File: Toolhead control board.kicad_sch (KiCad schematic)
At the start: 28 parts, among them J1 Conn_01x02_Pin, J2 Conn_01x02_Pin, J3 Conn_01x06_Pin, J4 Conn_01x02_Pin, J5 Conn_01x02_Pin, J6 Conn_01x02_Pin, Q1 AS3400, Q2 AS3400, Q3 AS3400, U1 ADXL345, U2 STM32F042G6Ux, Y1 8MHz

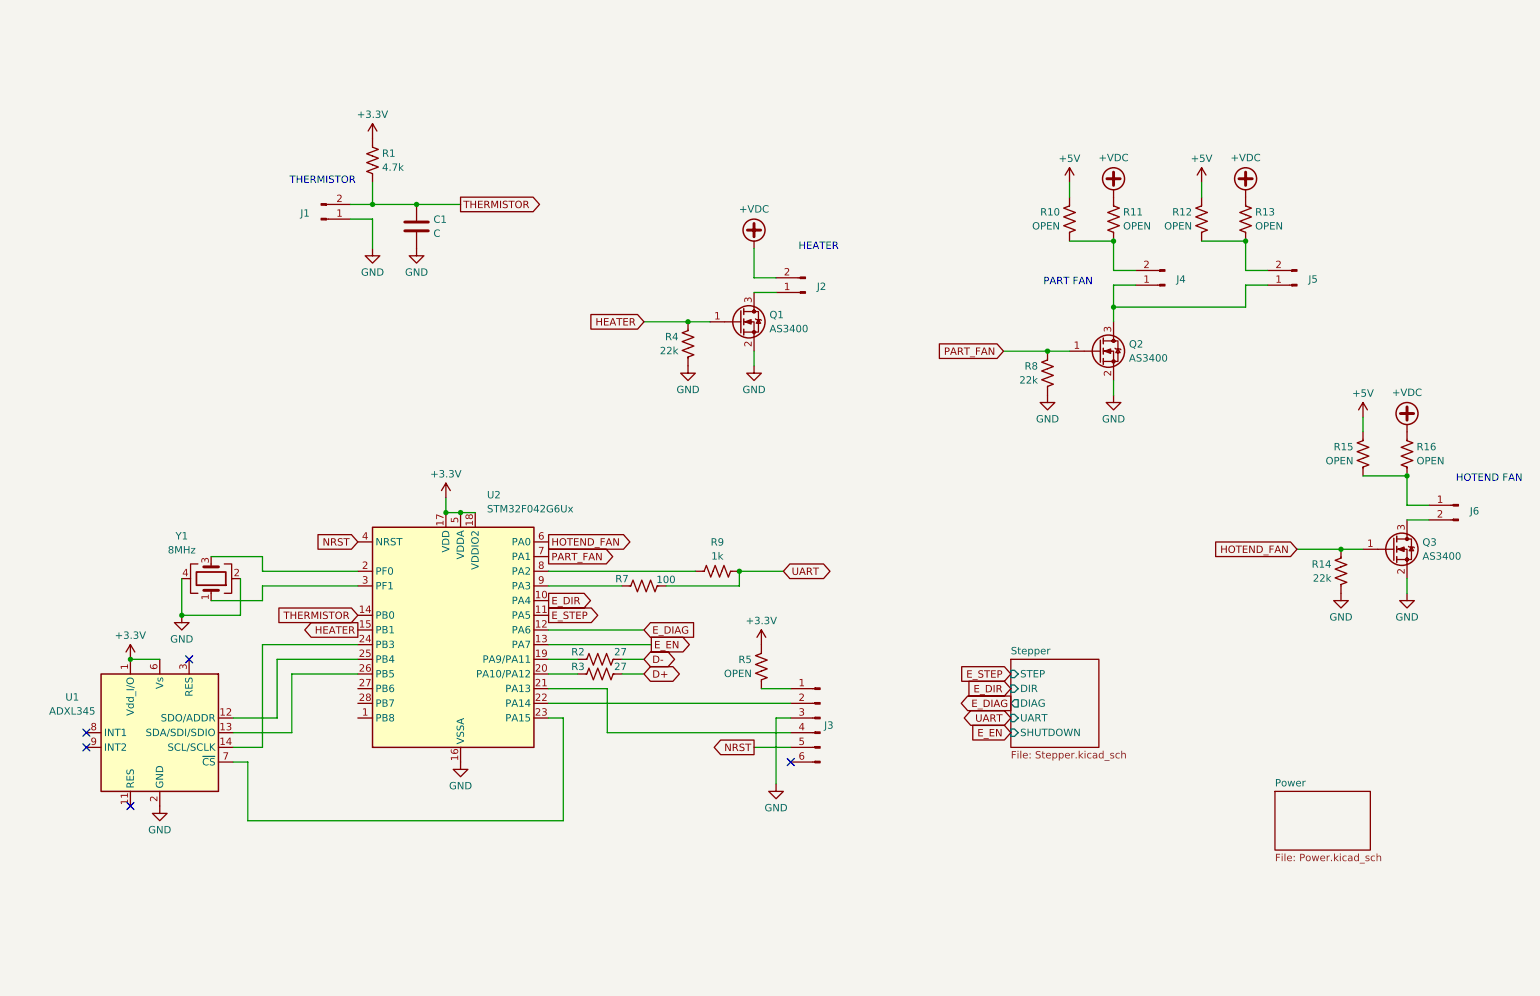
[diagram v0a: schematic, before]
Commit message: Rev1. Uart interface
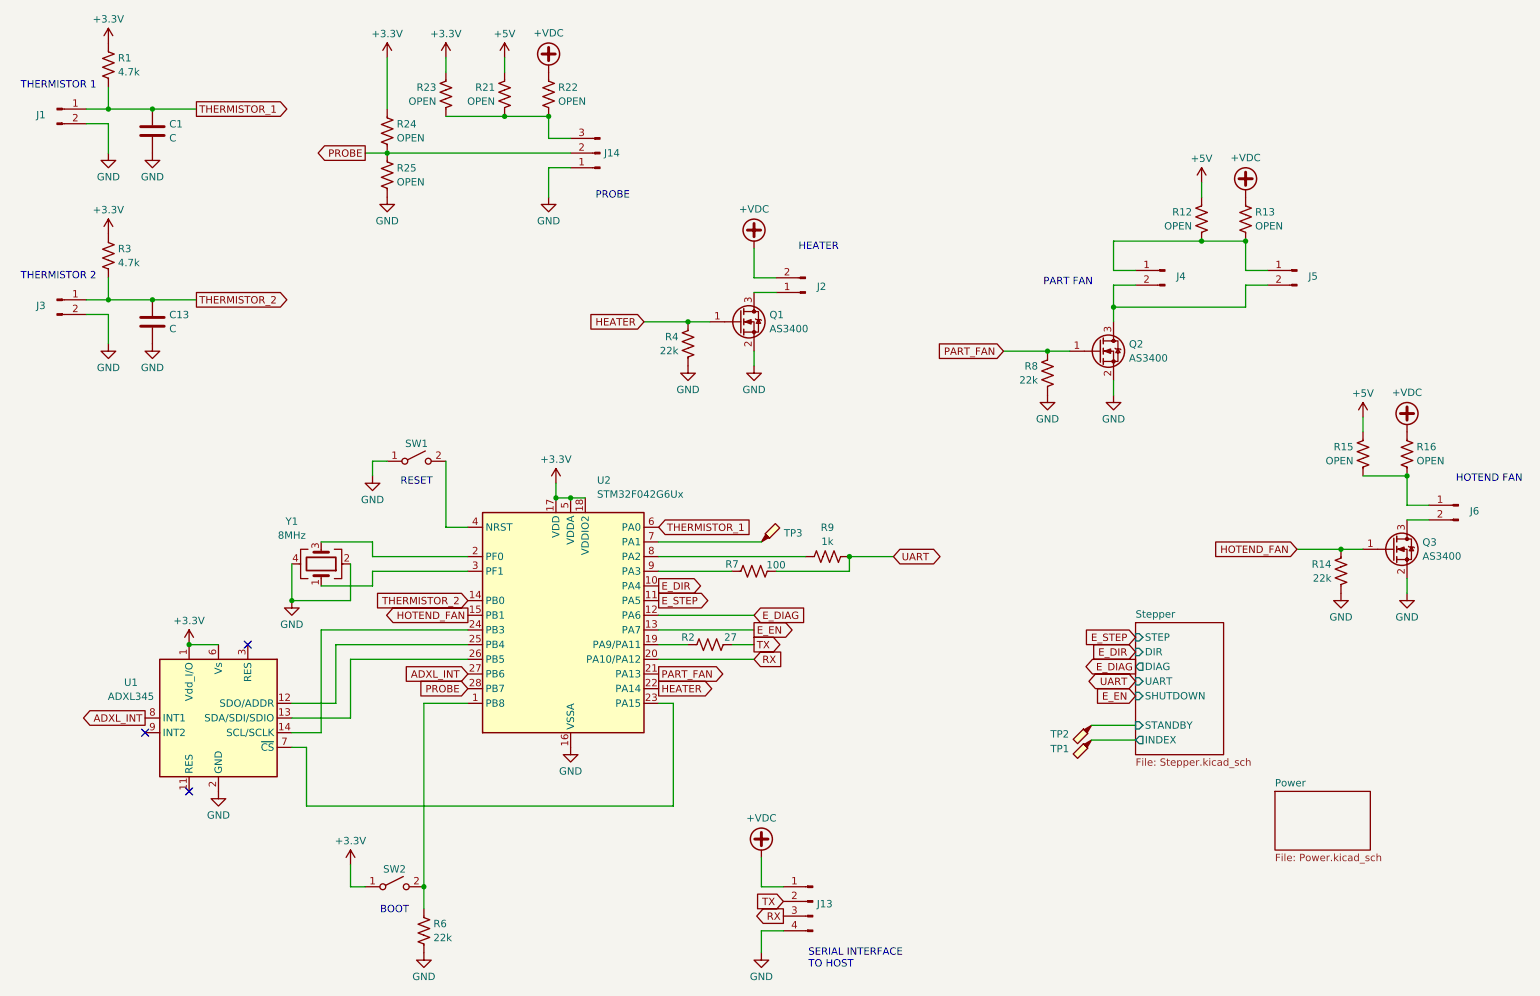
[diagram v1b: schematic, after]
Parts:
- removed J3: Conn_01x06_Pin, Connector_PinHeader_2.54mm:PinHeader_1x06_P2.54mm_Vertical, symbol Connector:Conn_01x06_Pin
- removed R10, R11, R5: OPEN, Resistor_SMD:R_0805_2012Metric, symbol Device:R_US
- added C13: C, Capacitor_SMD:C_0805_2012Metric, symbol Device:C
- added J13: Conn_01x04_Male, Connector_JST:JST_XH_B4B-XH-A_1x04_P2.50mm_Vertical, symbol Connector:Conn_01x04_Male
- added J14: Conn_01x04_Male, Connector_JST:JST_XH_B4B-XH-A_1x04_P2.50mm_Vertical, symbol Connector:Conn_01x03_Pin
- added J3: Conn_01x02_Pin, Connector_JST:JST_XH_S2B-XH-A-1_1x02_P2.50mm_Horizontal, symbol Connector:Conn_01x02_Pin
- added R21, R22, R23, R24, R25: OPEN, Resistor_SMD:R_0805_2012Metric, symbol Device:R_US
- added R6: 22k, Resistor_SMD:R_0805_2012Metric, symbol Device:R_US
- added SW1, SW2: SW_SPST, Button_Switch_SMD:SW_SPST_B3U-1000P, symbol Switch:SW_SPST
- added TP1, TP2, TP3: TestPoint_Probe, TestPoint:TestPoint_Pad_D1.0mm, symbol Connector:TestPoint_Probe
- R3: value 27 -> 4.7k
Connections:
- net +3.3V: now also R3.1, R23.1, R24.1, SW2.1 (A)
- net +5V: now also R21.1
- net +VDC: now also J13.1 (Pin_1), R22.1
- net GND: now also J1.2 (Pin_2), C13.2, J13.4 (Pin_4), J14.1 (Pin_1), J3.2 (Pin_2), R25.2, R6.2, SW1.1 (A); no longer J1.1 (Pin_1)
- net HEATER: now also U2.22 (PA14); no longer U2.15 (PB1)
- net HOTEND_FAN: now also U2.15 (PB1); no longer U2.6 (PA0)
- net PART_FAN: now also U2.21 (PA13); no longer U2.7 (PA1)
- net at J4.1 (Pin_1), J5.1 (Pin_1): now also R12.2, R13.2; no longer Q2.3 (D)
- net RX: now reaches U2.20 (PA10/PA12)
- net RX: now also J13.3 (Pin_3); no longer R3.1
- net ADXL_INT: now reaches U1.8 (INT1)
- net ADXL_INT: now also U2.27 (PB6)
- net at J4.2 (Pin_2): now also J5.2 (Pin_2), Q2.3 (D)
- net at U2.1 (PB8): now also R6.1, SW2.2 (B)
- net PROBE: now reaches U2.28 (PB7)
- net PROBE: now also J14.2 (Pin_2), R24.2, R25.1
- net D+ renamed THERMISTOR_2
- net THERMISTOR_2: now also U2.14 (PB0), C13.1, J3.1 (Pin_1)
- net D- renamed TX
- net TX: now also J13.2 (Pin_2)
- net NRST: no longer names the net of U2.4 (NRST)
- net NRST: now also SW1.2 (B)
- net THERMISTOR renamed THERMISTOR_1
- net THERMISTOR_1: now also J1.1 (Pin_1), U2.6 (PA0); no longer J1.2 (Pin_2), U2.14 (PB0)
- new net: J14.3 (Pin_3), R21.2, R22.2, R23.2
- new net: TP3.1, U2.7 (PA1)
- new net Stepper/INDEX: TP1.1
- new net Stepper/STANDBY: TP2.1
- no-connect marks 5 -> 3
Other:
- sheet Stepper ports: added INDEX, STANDBY; removed none
- note added: "BOOT"
- note added: "PROBE"
- note added: "RESET"
- note added: "SERIAL INTERFACE TO HOST"
- note added: "THERMISTOR 1"
- note added: "THERMISTOR 2"
- note removed: "THERMISTOR"
- moved on the sheet: C1, J1, J4, J5, R1, R2, R7, R9, U1, U2, Y1
